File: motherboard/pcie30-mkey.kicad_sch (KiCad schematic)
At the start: 50 parts, among them IC1 PI6C557-05BLE, J15 Bus_M.2_Socket_M, U20 TPS54331DR, U21 AP2127K-3.3, Y1 25MHz

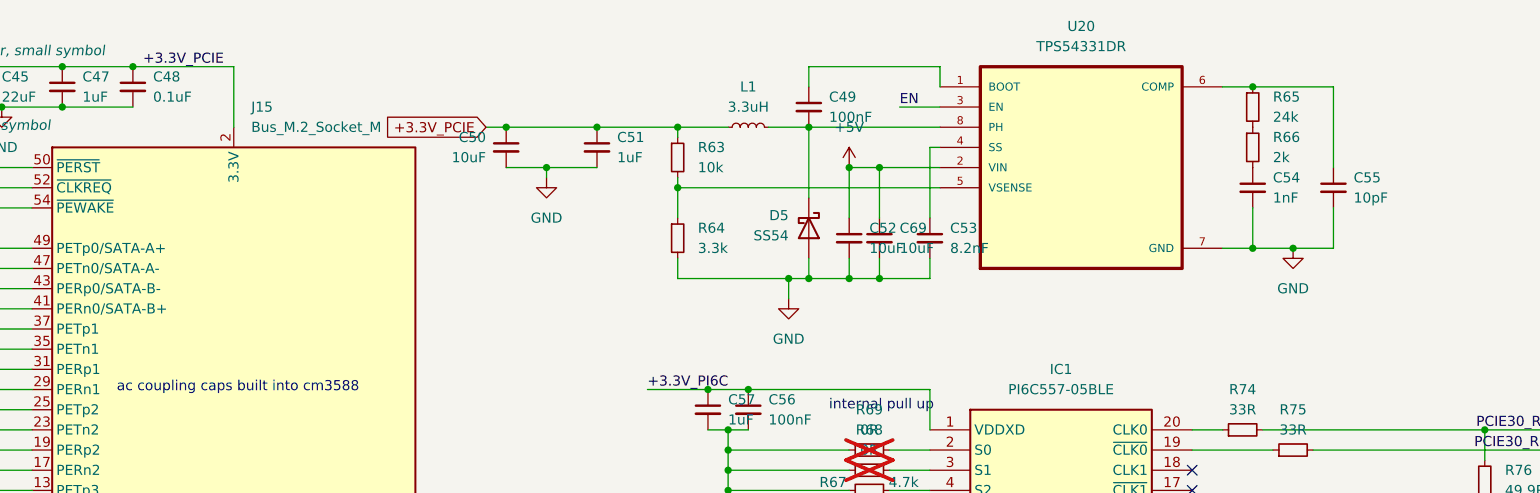
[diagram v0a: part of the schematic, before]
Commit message: v0.2 layout
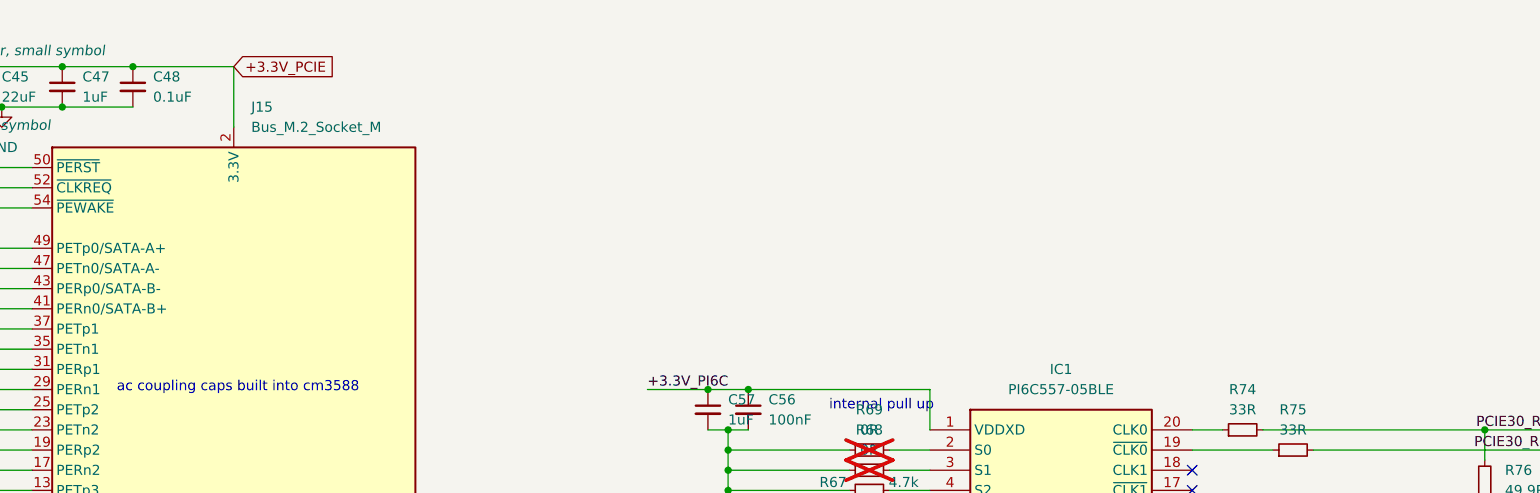
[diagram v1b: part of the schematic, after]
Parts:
- removed C49: 100nF, Capacitor_SMD:C_0402_1005Metric, symbol Device:C_Small
- removed C50, C52, C69: 10uF, Capacitor_SMD:C_0603_1608Metric, symbol Device:C_Small
- removed C51: 1uF, Capacitor_SMD:C_0402_1005Metric, symbol Device:C_Small
- removed C53: 8.2nF, Capacitor_SMD:C_0402_1005Metric, symbol Device:C_Small
- removed C54: 1nF, Capacitor_SMD:C_0402_1005Metric, symbol Device:C_Small
- removed C55: 10pF, Capacitor_SMD:C_0402_1005Metric, symbol Device:C_Small
- removed D5: SS54, Diode_SMD:D_SMA, symbol Device:D_Schottky
- removed L1: 3.3uH, Inductor_SMD:L_Vishay_IHLP-1616, symbol Device:L_Small
- removed R63: 10k, Resistor_SMD:R_0402_1005Metric, symbol Device:R_Small
- removed R64: 3.3k, Resistor_SMD:R_0402_1005Metric, symbol Device:R_Small
- removed R65: 24k, Resistor_SMD:R_0402_1005Metric, symbol Device:R_Small
- removed R66: 2k, Resistor_SMD:R_0402_1005Metric, symbol Device:R_Small
- removed U20: TPS54331DR, TPS54331DR:SOIC127P599X175-8N, symbol TPS54331DR:TPS54331DR
